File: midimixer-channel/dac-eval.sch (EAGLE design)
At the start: 20 parts, among them IC1 NE5534AD

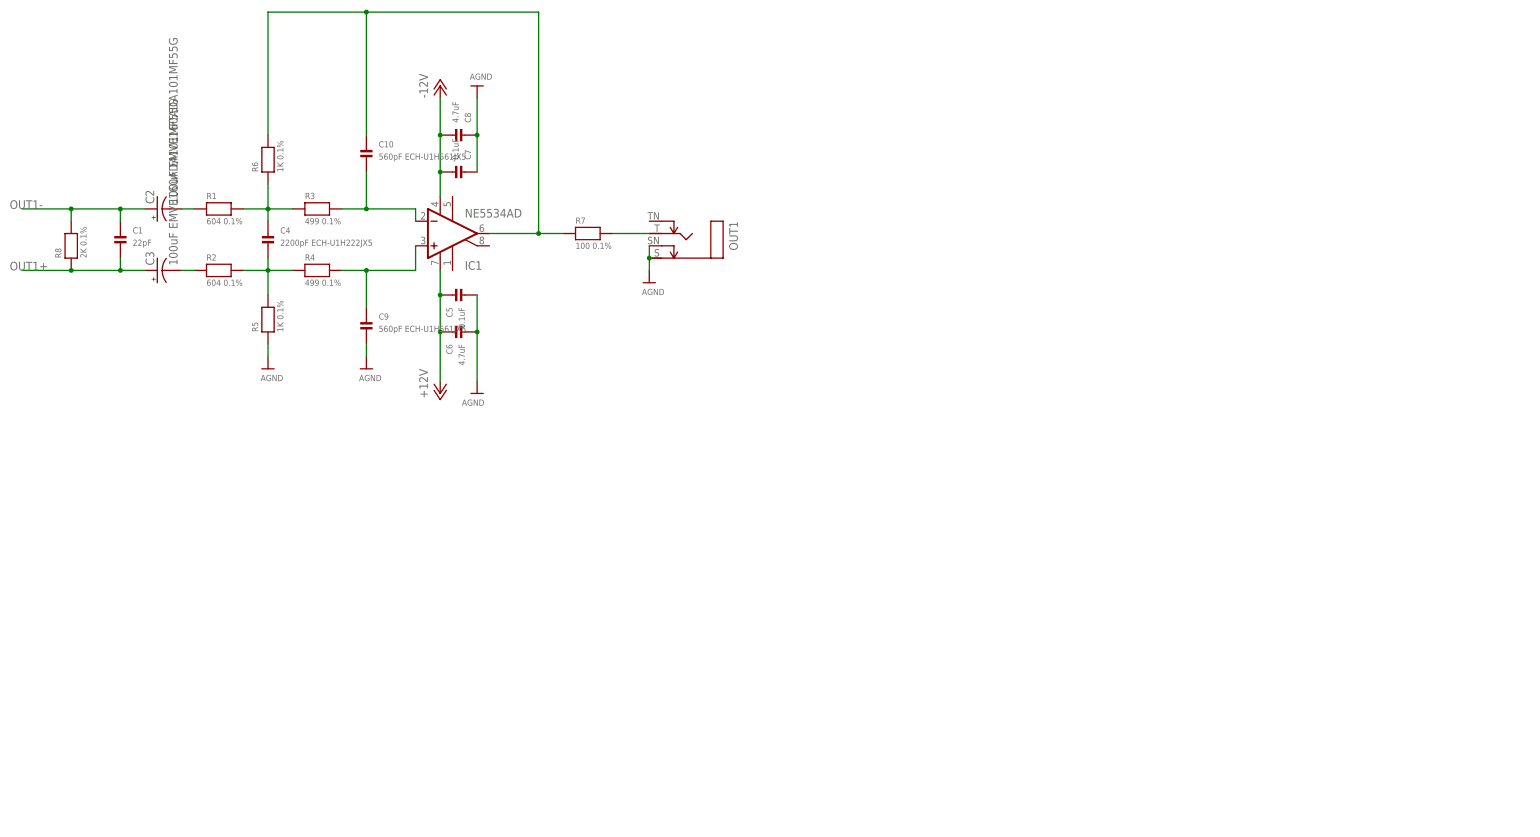
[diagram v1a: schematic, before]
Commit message: dac wip
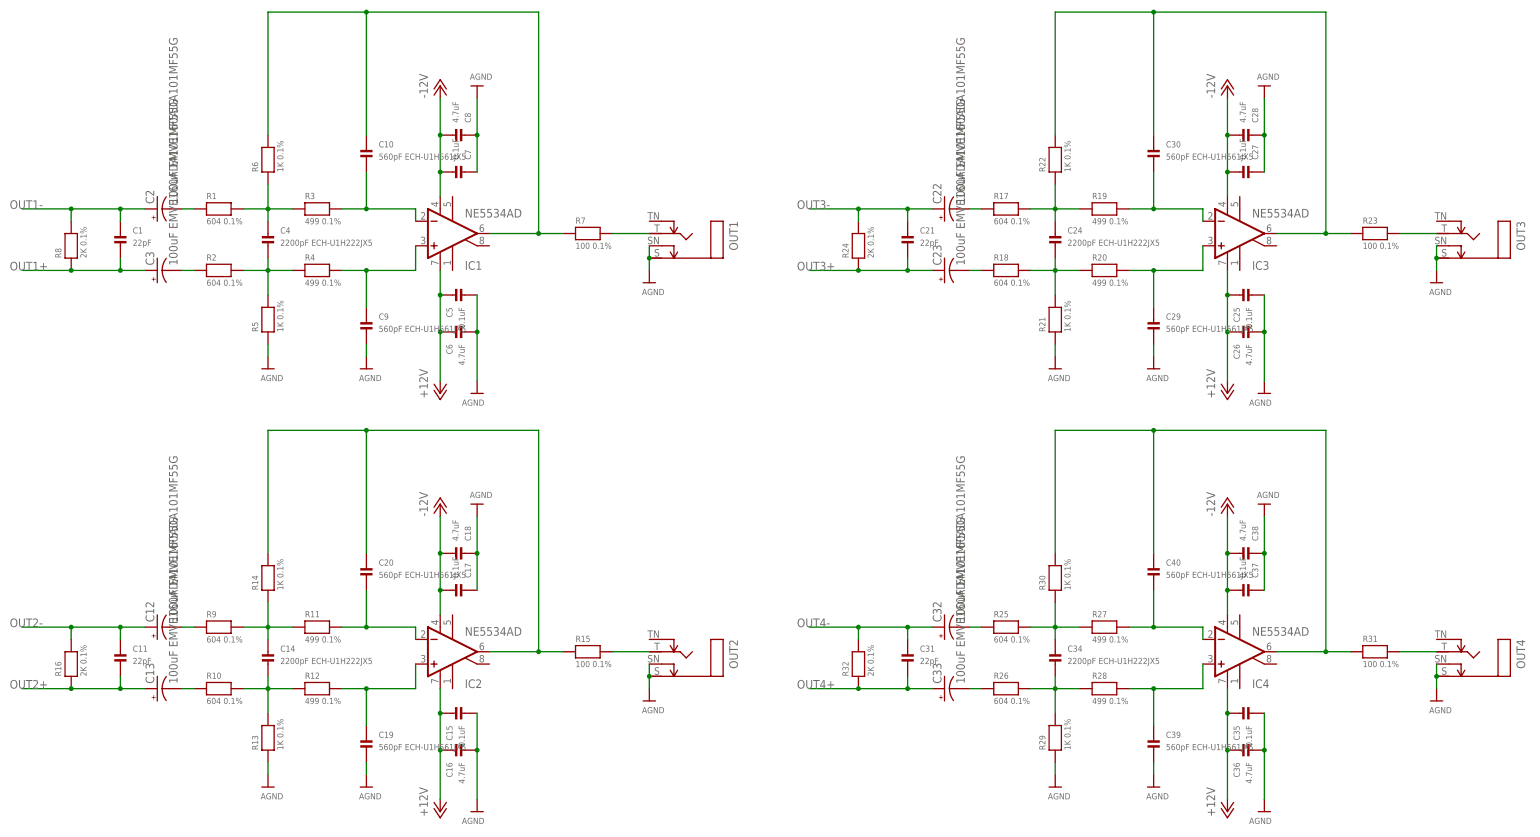
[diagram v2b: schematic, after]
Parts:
- added C11, C21, C31: 22pF, microbuilder:CAP_CERAMIC0603
- added C12, C13, C22, C23, C32, C33: 100uF EMVE160ADA101MF55G, SparkFun-Capacitors:CAP_POLD
- added C14, C24, C34: 2200pF ECH-U1H222JX5, microbuilder:CAP_CERAMIC0805
- added C15, C17, C25, C27, C35, C37: 0.1uF, microbuilder:CAP_CERAMIC0603
- added C16, C18, C26, C28, C36, C38: 4.7uF, microbuilder:CAP_CERAMIC0603
- added C19, C20, C29, C30, C39, C40: 560pF ECH-U1H561JX5, microbuilder:CAP_CERAMIC0805
- added IC2, IC3, IC4: NE5534AD, linear:NE5534AD
- added OUT2, OUT3, OUT4: NMJ4HFD2, pl-jacks:MONOSWS
- added R10, R17, R18, R25, R26, R9: 604 0.1%, microbuilder:RESISTOR0603
- added R11, R12, R19, R20, R27, R28: 499 0.1%, microbuilder:RESISTOR0603
- added R13, R14, R21, R22, R29, R30: 1K 0.1%, microbuilder:RESISTOR0603
- added R15, R23, R31: 100 0.1%, microbuilder:RESISTOR0603
- added R16, R24, R32: 2K 0.1%, microbuilder:RESISTOR0603
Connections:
- new net N$1: C12.-, R9.1
- new net N$11: C14.P$1, R11.1, R14.1, R9.2
- new net N$13: C19.P$1, IC2.+IN, R12.2
- new net N$14: C20.P$2, IC2.-IN, R11.2
- new net N$15: C20.P$1, IC2.OUT, R14.2, R15.1
- new net N$16: OUT2.T, R15.2
- new net N$17: C22.-, R17.1
- new net N$18: C23.-, R18.1
- new net N$19: C24.P$2, R18.2, R20.1, R21.2
- new net N$2: C13.-, R10.1
- new net N$20: C24.P$1, R17.2, R19.1, R22.1
- new net N$21: C29.P$1, IC3.+IN, R20.2
- new net N$22: C30.P$2, IC3.-IN, R19.2
- new net N$23: C30.P$1, IC3.OUT, R22.2, R23.1
- new net N$24: OUT3.T, R23.2
- new net N$25: C32.-, R25.1
- new net N$26: C33.-, R26.1
- new net N$27: C34.P$2, R26.2, R28.1, R29.2
- new net N$28: C34.P$1, R25.2, R27.1, R30.1
- new net N$29: C39.P$1, IC4.+IN, R28.2
- new net N$30: C40.P$2, IC4.-IN, R27.2
- new net N$31: C40.P$1, IC4.OUT, R30.2, R31.1
- new net N$32: OUT4.T, R31.2
- new net N$7: C14.P$2, R10.2, R12.1, R13.2
- new net OUT2+: C11.P$2, C13.+, R16.1
- new net OUT2-: C11.P$1, C12.+, R16.2
- new net OUT3+: C21.P$2, C23.+, R24.1
- new net OUT3-: C21.P$1, C22.+, R24.2
- new net OUT4+: C31.P$2, C33.+, R32.1
- new net OUT4-: C31.P$1, C32.+, R32.2
- net +12V: now also C15.P$1, C16.P$1, C25.P$1, C26.P$1, C35.P$1, C36.P$1, IC2.V+, IC3.V+, IC4.V+
- net -12V: now also C17.P$2, C18.P$2, C27.P$2, C28.P$2, C37.P$2, C38.P$2, IC2.V-, IC3.V-, IC4.V-
- net AGND: now also C15.P$2, C16.P$2, C17.P$1, C18.P$1, C19.P$2, C25.P$2, C26.P$2, C27.P$1, C28.P$1, C29.P$2, C35.P$2, C36.P$2, C37.P$1, C38.P$1, C39.P$2, OUT2.S, OUT2.SN, OUT3.S, OUT3.SN, OUT4.S, OUT4.SN, R13.1, R21.1, R29.1
